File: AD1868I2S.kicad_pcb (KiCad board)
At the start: 2 copper layers, 41.9 x 27.9 mm, 16 parts, among them J1 054986, J2 JTAG, J3 I2S, SW1 MODE, U1 EPM3064A(TQFP), U2 AMS1117-3.3, X1 22.5792MHz

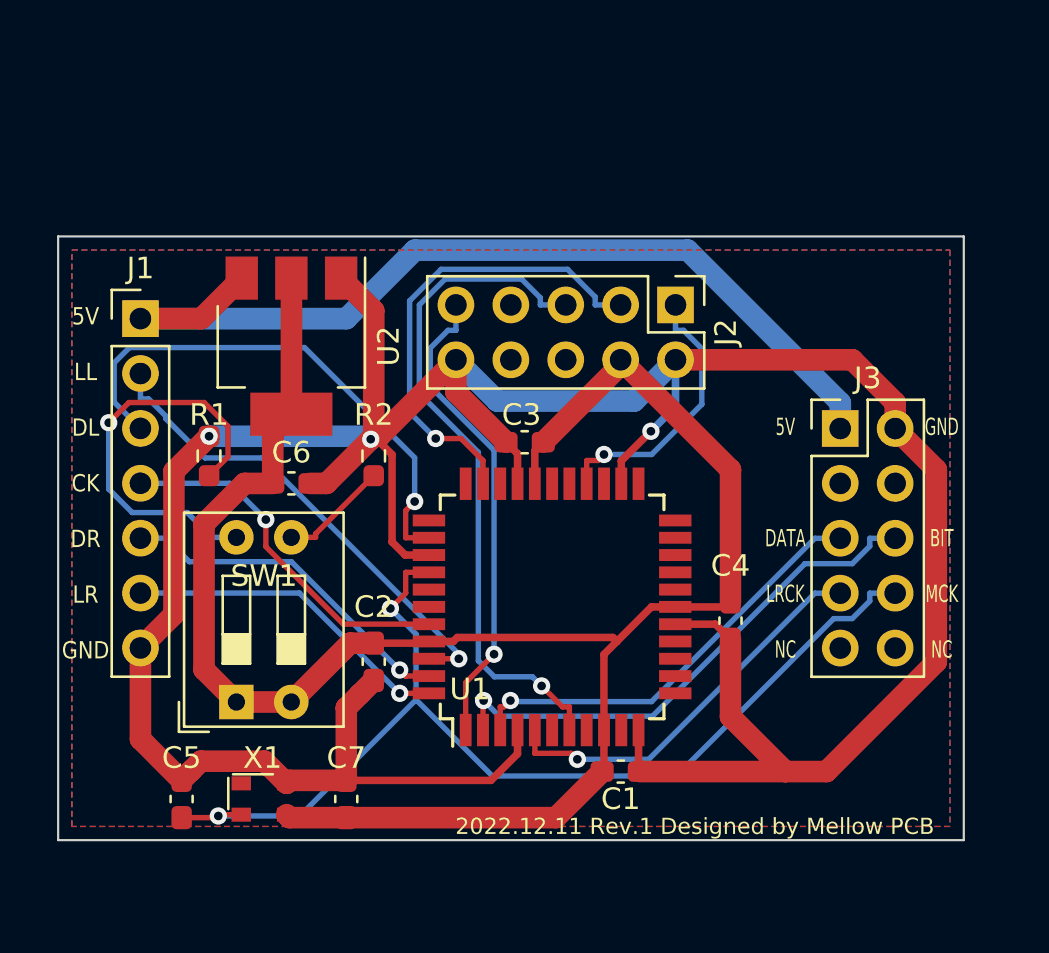
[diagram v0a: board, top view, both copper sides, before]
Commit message: update pcb to rev2
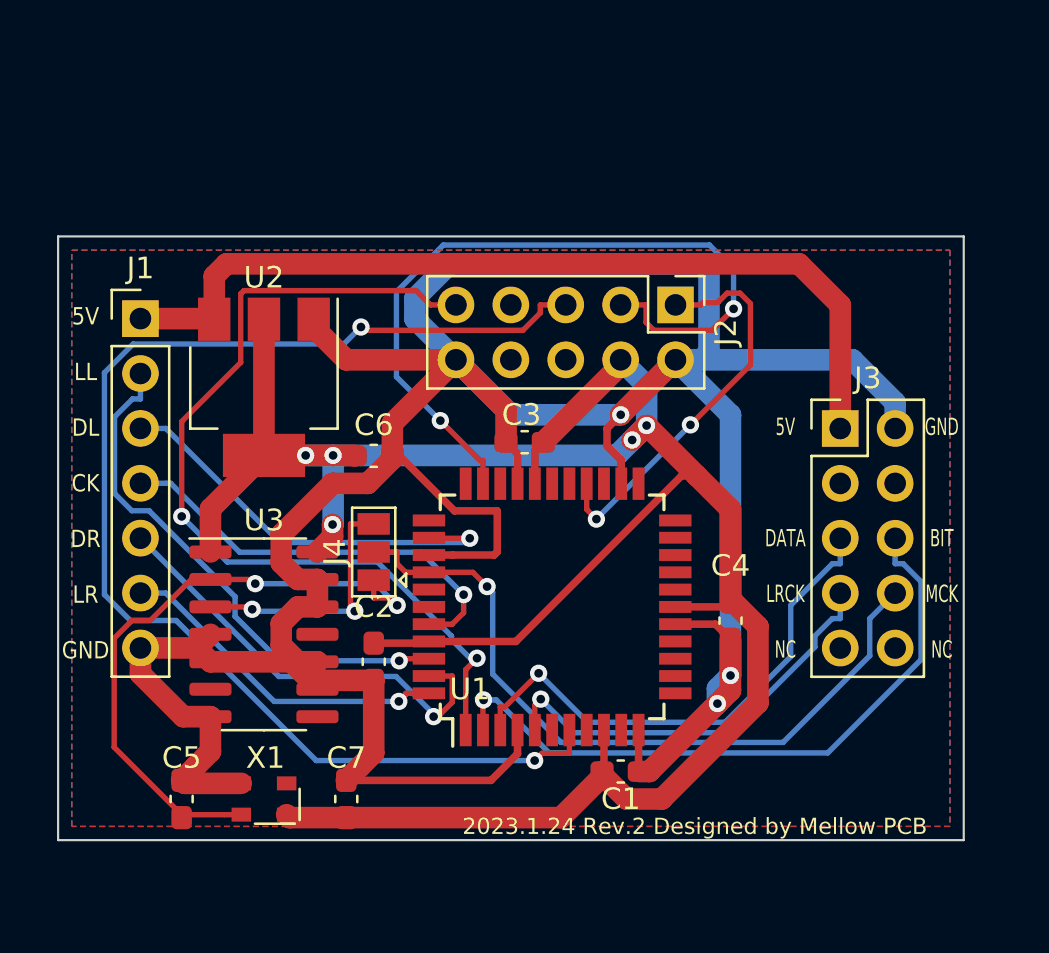
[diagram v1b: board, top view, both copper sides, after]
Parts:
- removed R1, R2: 10k, Resistor_SMD:R_0603_1608Metric_Pad0.98x0.95mm_HandSolder
- removed SW1: MODE, Button_Switch_THT:SW_DIP_SPSTx02_Slide_9.78x7.26mm_W7.62mm_P2.54mm
- added J4: Conn_01x03, Jumper:SolderJumper-3_P1.3mm_Open_Pad1.0x1.5mm, F.Cu at (84.5, 100.3)
- added U3: 74HC86, Package_SO:SOIC-14_3.9x8.7mm_P1.27mm, F.Cu at (79.4, 104.1)
- moved C6 4.02 mm to (84.5, 95.9)
- moved U2 2.29 mm to (79.4, 92.7)
- turned X1 to 180 degrees
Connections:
- C5 pad 1: /I2S_MCK -> /XCK
- U1 pad 10: /DIP2 -> unconnected-(U1-Pad10)
- U1 pad 8: /DIP1 -> unconnected-(U1-Pad8)
- X1 pad 3: /I2S_MCK -> /XCK
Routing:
- net /XCK: track 0.00 -> 29.1 mm, vias 0 -> 2
- net /TMS: track 31.7 -> 59.2 mm, vias 1 -> 2
- net +3.3V: track 90.3 -> 112.2 mm, vias 0 -> 5
- net GND: track 152.0 -> 171.7 mm
- net /TDI: track 22.1 -> 41.7 mm, vias 1 -> 2
- net Net-(R1-Pad1): track 18.9 -> 0.00 mm, vias 1 -> 0
- net /I2S_MCK: track 49.3 -> 34.2 mm, vias 2 -> 1
- net /TDO: track 21.8 -> 36.0 mm, vias 1 -> 2
- net /XCK_X: track 0.00 -> 12.0 mm, vias 0 -> 2
- net /I2S_CLK: track 24.3 -> 30.8 mm
- net /TCK: track 12.8 -> 18.6 mm, vias 1 -> 2
- net /DL: track 24.8 -> 19.4 mm
- net Net-(R2-Pad1): track 5.09 -> 0.00 mm
- net /DR: track 16.0 -> 20.5 mm
- net /I2S_DT: track 20.1 -> 24.0 mm
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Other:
- board text added: "2023.1.24 Rev.2 Designed by Mellow PCB"
- board text removed: "2022.12.11 Rev.1 Designed by Mellow PCB"

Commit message: rev3
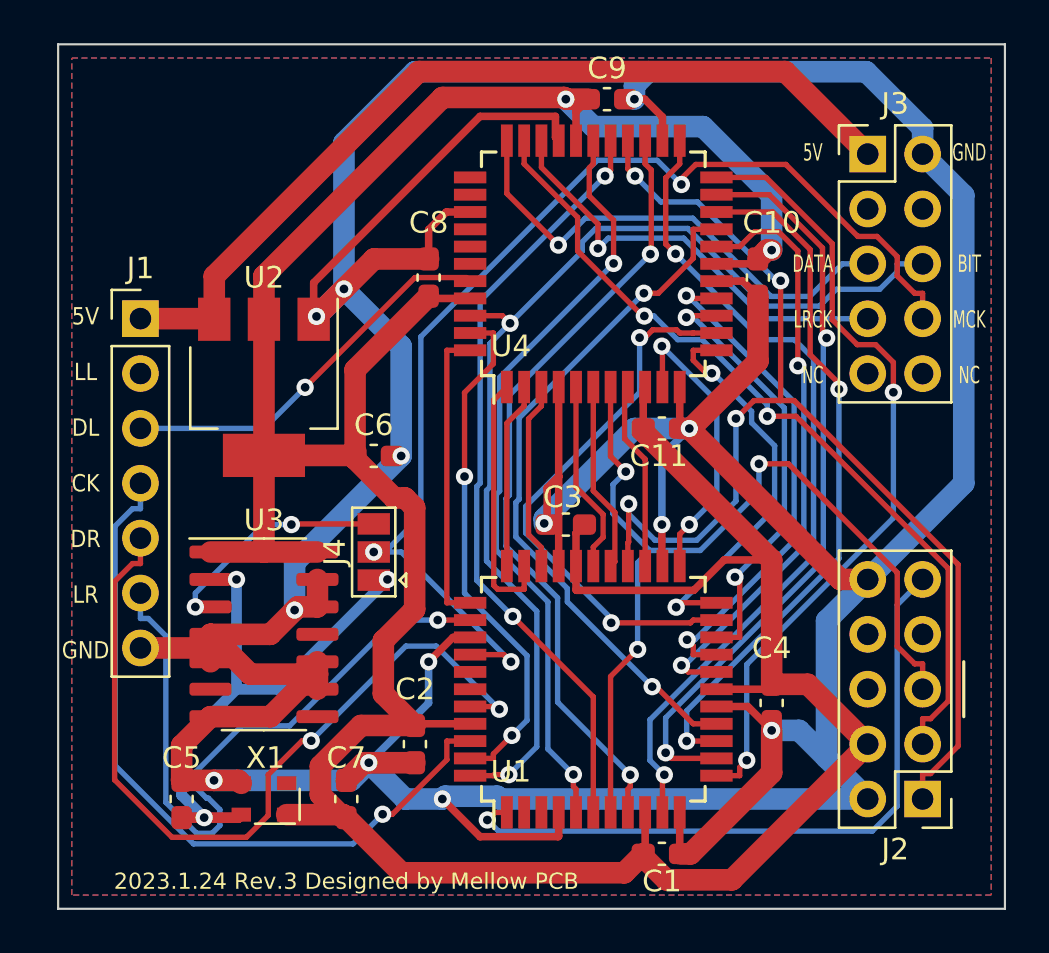
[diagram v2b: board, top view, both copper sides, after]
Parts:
- added C10: 0.1uF, Capacitor_SMD:C_0603_1608Metric_Pad1.08x0.95mm_HandSolder, F.Cu at (102.2, 87.6)
- added C11: 0.1uF, Capacitor_SMD:C_0603_1608Metric_Pad1.08x0.95mm_HandSolder, F.Cu at (97.8, 94.6)
- added C8: 0.1uF, Capacitor_SMD:C_0603_1608Metric_Pad1.08x0.95mm_HandSolder, F.Cu at (87.0, 87.6)
- added C9: 0.1uF, Capacitor_SMD:C_0603_1608Metric_Pad1.08x0.95mm_HandSolder, F.Cu at (95.2, 79.4)
- added U4: EPM3064A(TQFP), Package_QFP:TQFP-44_10x10mm_P0.8mm, F.Cu at (94.6, 87.0)
- moved J2 25.6 mm to (109.9, 111.8), turned to 180 degrees
- moved J3 12.8 mm to (107.3, 81.9)
- moved C1 4.26 mm to (97.8, 114.3)
- moved C2 4.26 mm to (86.4, 109.2)
- moved C3 4.26 mm to (93.3, 99.1)
- moved C4 4.26 mm to (102.9, 107.3)
- moved U1 4.26 mm to (94.6, 106.7)
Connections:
- U1 pad 10: unconnected-(U1-Pad10) -> /DR3
- U1 pad 12: unconnected-(U1-Pad12) -> /DR4
- U1 pad 13: unconnected-(U1-Pad13) -> /DR5
- U1 pad 14: unconnected-(U1-Pad14) -> /DR6
- U1 pad 15: unconnected-(U1-Pad15) -> /DR7
- U1 pad 18: unconnected-(U1-Pad18) -> /DR8
- U1 pad 19: unconnected-(U1-Pad19) -> /DR9
- U1 pad 2: /I2S_CLK -> unconnected-(U1-Pad2)
- U1 pad 20: unconnected-(U1-Pad20) -> /DR10
- U1 pad 21: unconnected-(U1-Pad21) -> /DR11
- U1 pad 22: unconnected-(U1-Pad22) -> /DR12
- U1 pad 23: unconnected-(U1-Pad23) -> /DR13
- U1 pad 25: unconnected-(U1-Pad25) -> /DR14
- U1 pad 27: unconnected-(U1-Pad27) -> /DR15
- U1 pad 28: unconnected-(U1-Pad28) -> /DR16
- U1 pad 3: /I2S_DT -> unconnected-(U1-Pad3)
- U1 pad 31: unconnected-(U1-Pad31) -> /DR17
- U1 pad 32: /TDO -> /TDX
- U1 pad 33: unconnected-(U1-Pad33) -> /AD_LP
- U1 pad 34: unconnected-(U1-Pad34) -> /LATCH
- U1 pad 35: /DL -> /LR
- U1 pad 40: /CK -> /DR
- U1 pad 42: /LL -> /CK
- U1 pad 43: /DR -> /SYNC_CLK
- U1 pad 44: /LR -> /I2S_CLK
- U1 pad 5: /I2S_LR -> /DR0
- U1 pad 6: unconnected-(U1-Pad6) -> /DR1
- U1 pad 8: unconnected-(U1-Pad8) -> /DR2
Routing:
- net GND: track 171.7 -> 270.7 mm, vias 3 -> 13
- net +3.3V: track 112.2 -> 166.7 mm, vias 5 -> 2
- net /DR3: track 0.00 -> 38.5 mm, vias 0 -> 2
- net /DR4: track 0.00 -> 36.9 mm, vias 0 -> 2
- net /DR2: track 0.00 -> 36.4 mm, vias 0 -> 2
- net /TCK: track 18.6 -> 55.0 mm, vias 2 -> 4
- net /DR1: track 0.00 -> 35.9 mm, vias 0 -> 2
- net /DR0: track 0.00 -> 35.4 mm, vias 0 -> 2
- net /DR5: track 0.00 -> 34.9 mm, vias 0 -> 2
- net /DR6: track 0.00 -> 32.7 mm, vias 0 -> 2
- net /DR7: track 0.00 -> 32.3 mm, vias 0 -> 2
- net /DR8: track 0.00 -> 27.9 mm, vias 0 -> 2
- net /DR11: track 0.00 -> 25.7 mm, vias 0 -> 2
- net /LL: track 24.6 -> 0.00 mm, vias 1 -> 0
- net /SYNC_CLK: track 0.00 -> 24.2 mm, vias 0 -> 2
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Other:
- board size 41.9 x 27.9 mm -> 43.8 x 40 mm
- board text added: "2023.1.24 Rev.3 Designed by Mellow PCB"
- board text removed: "2023.1.24 Rev.2 Designed by Mellow PCB"
